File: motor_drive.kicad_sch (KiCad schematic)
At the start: 15 parts, among them U1 DRV8316RRGFR

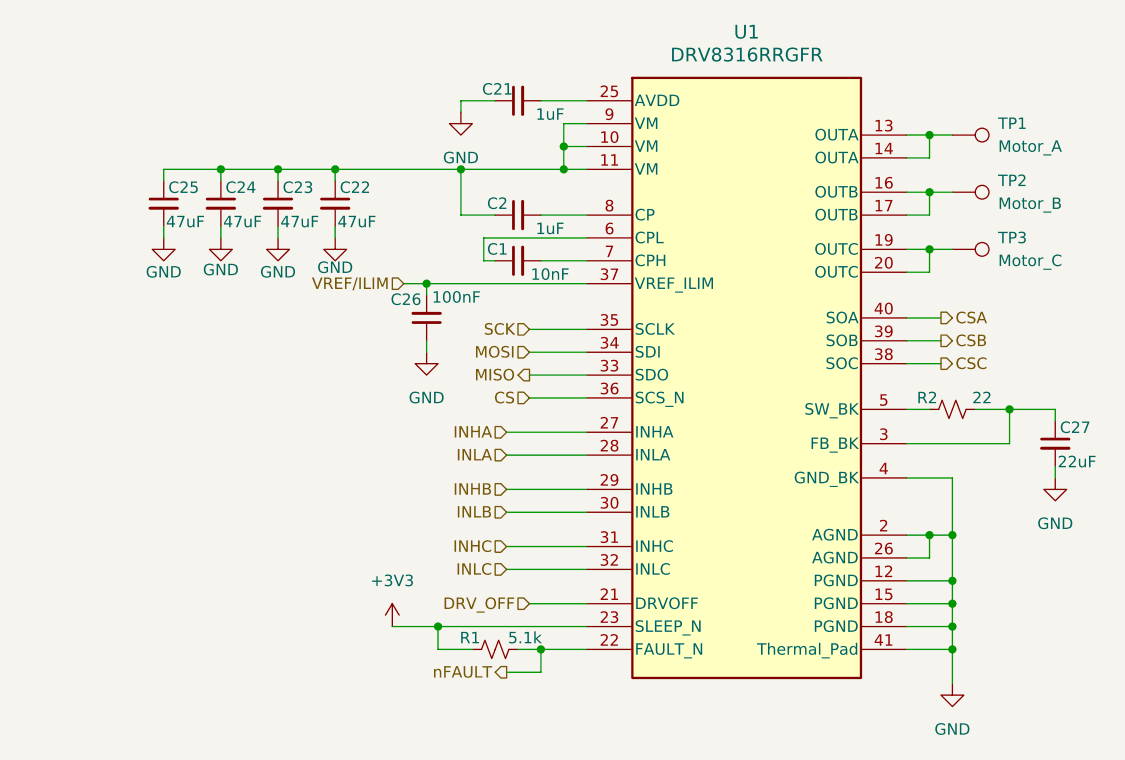
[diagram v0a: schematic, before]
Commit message: m2003 drive
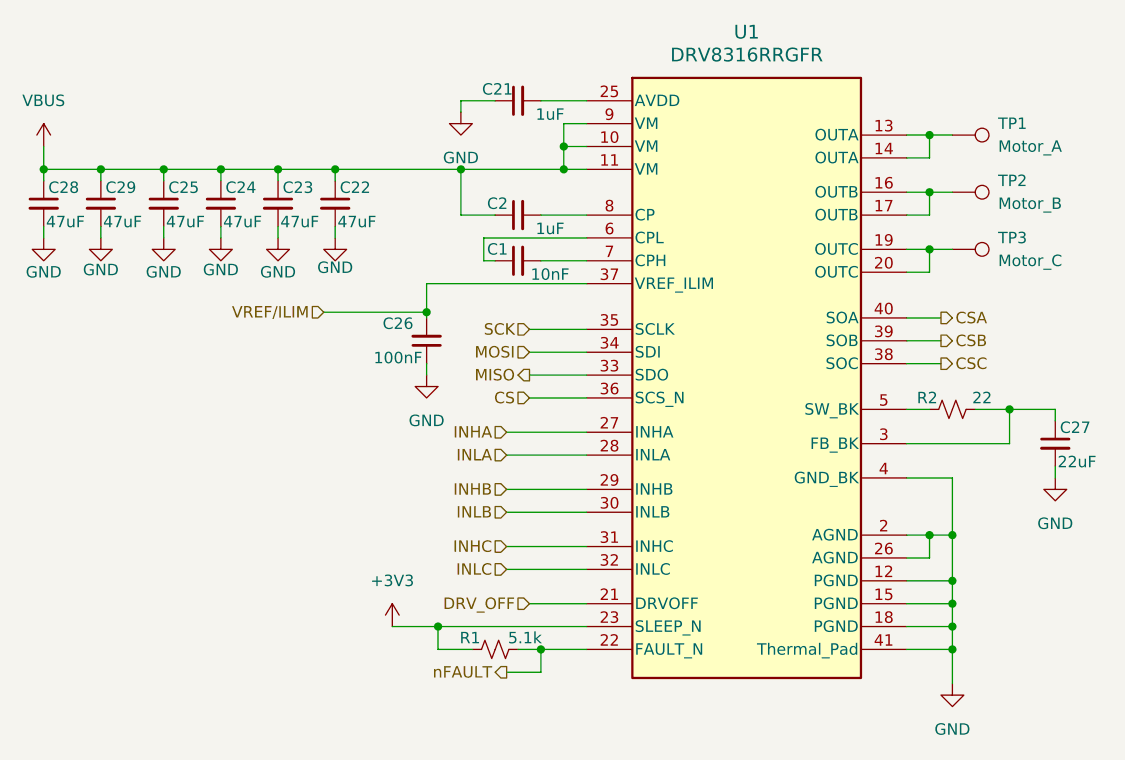
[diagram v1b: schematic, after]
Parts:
- added C28, C29: 47uF, Capacitor_SMD:C_0805_2012Metric, symbol Device:C_Small
- U1: footprint MSic:RGF0040E-MFG -> DRV8316:drv
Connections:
- net GND: now also C28.2, C29.2
- net VBUS: now reaches C2.1, C22.1, C23.1, C24.1, C25.1, U1.10 (VM), U1.11 (VM), U1.9 (VM)
- net VBUS: now also C28.1, C29.1
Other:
- moved on the sheet: C26
